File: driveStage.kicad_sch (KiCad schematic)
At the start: 45 parts

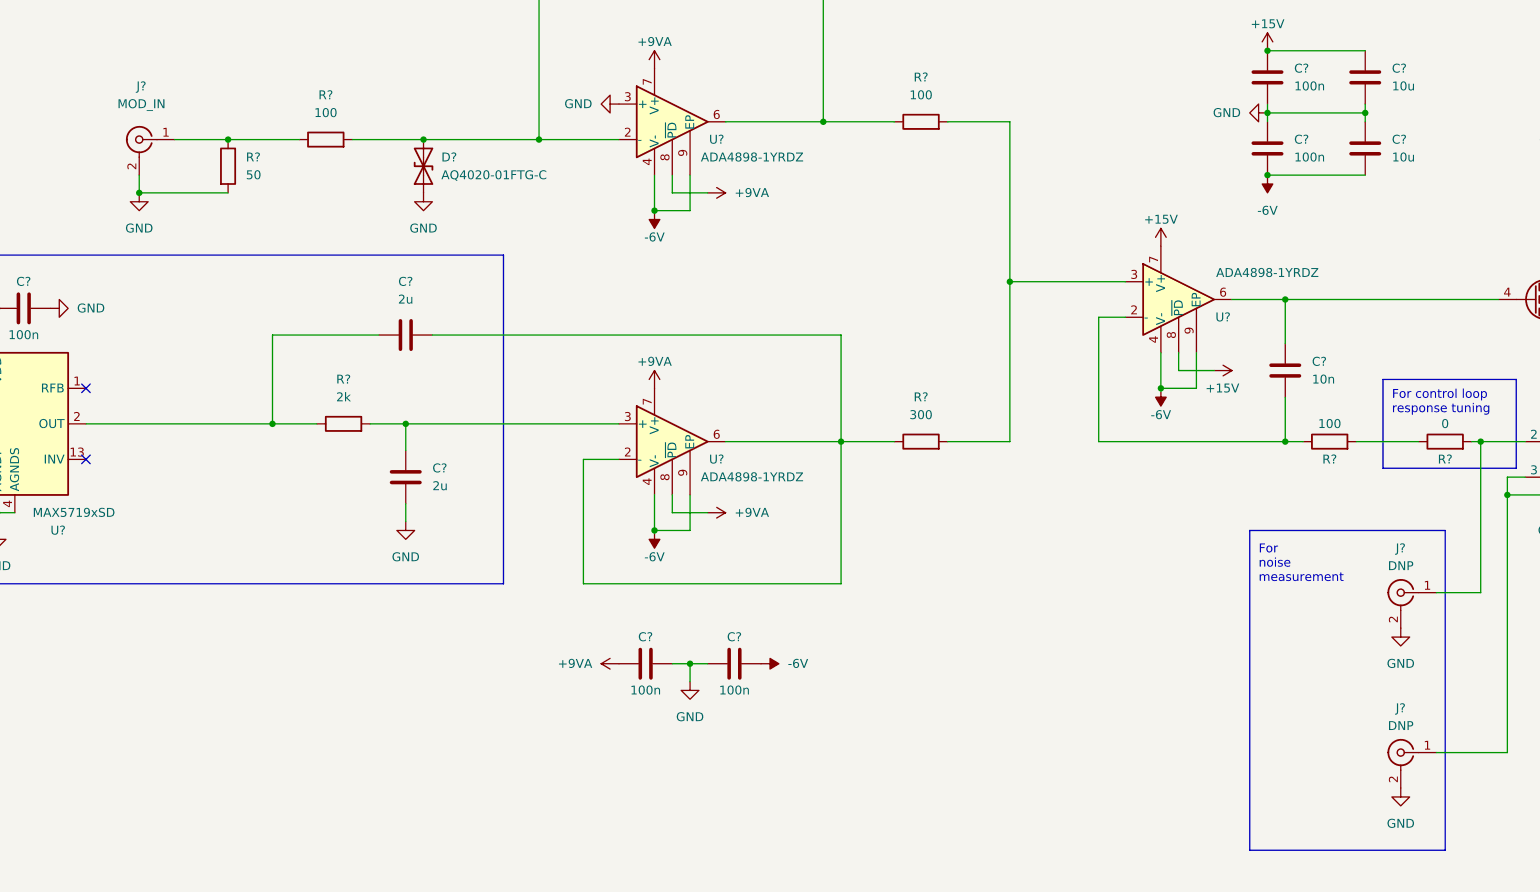
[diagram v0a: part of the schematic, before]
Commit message: add PoE
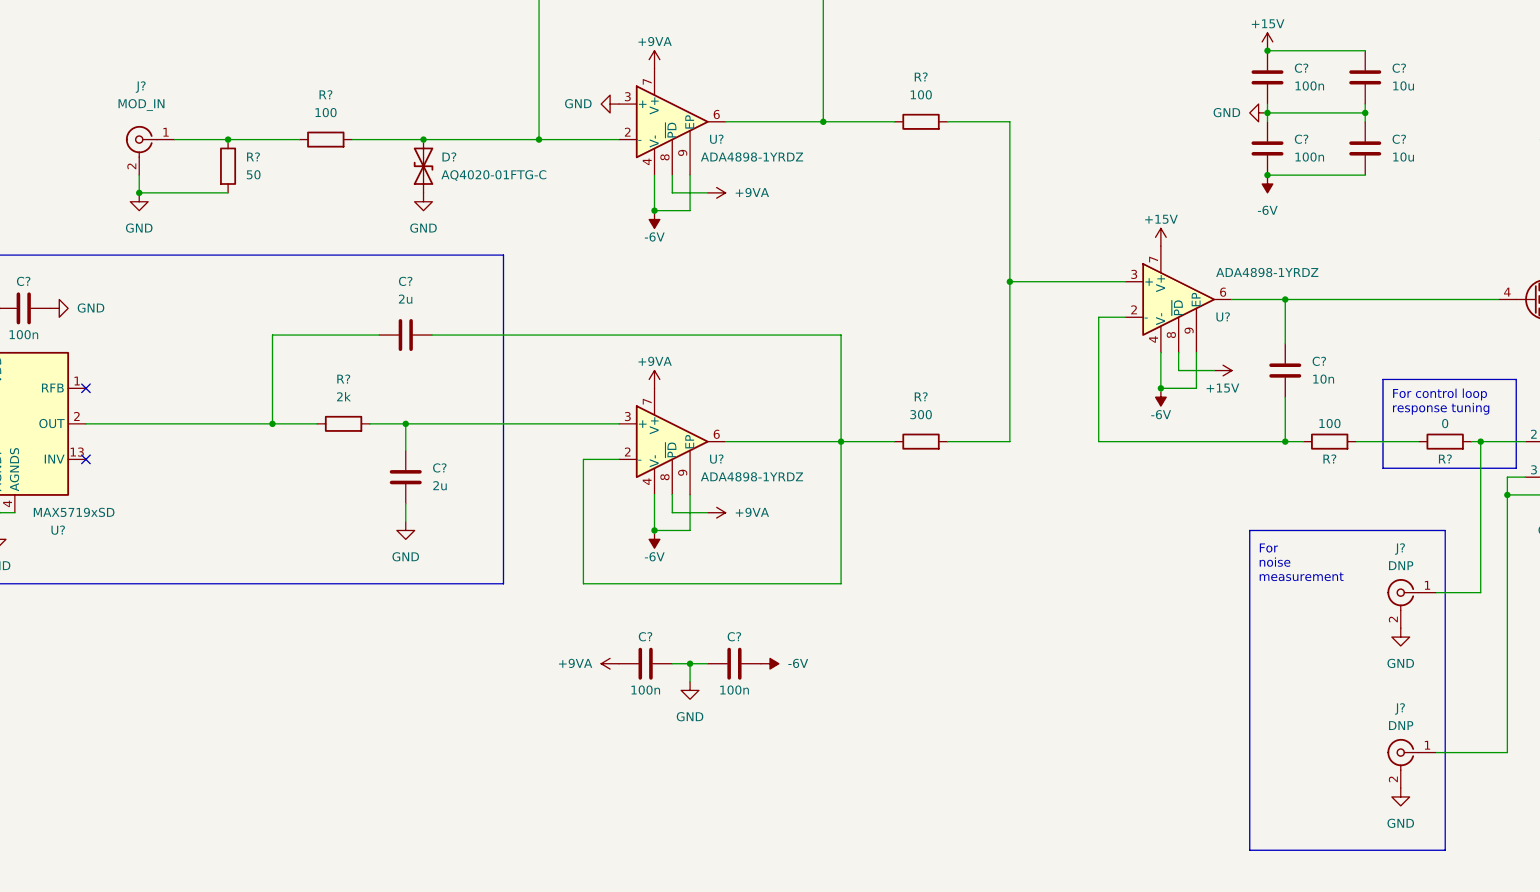
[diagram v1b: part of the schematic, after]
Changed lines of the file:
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@@
       (effects (font (size 1.27 1.27)) hide)
     )
-    (pin "1")
-    (pin "2")
-    (pin "3")
     (pin "5")
     (pin "6")
     (pin "7")
-    (pin "4")
-    (pin "8")
   )
   (symbol (lib_id "kirdy:RS8552") (at 339.09 208.28 0) (mirror y) (unit 1)
@@
     (pin "2")
     (pin "3")
-    (pin "5")
-    (pin "6")
-    (pin "7")
-    (pin "4")
-    (pin "8")
   )
   (symbol (lib_id "power:GND") (at 96.52 99.06 180) (unit 1)
@@
       (effects (font (size 1.27 1.27)) hide)
     )
-    (pin "1")
-    (pin "2")
-    (pin "3")
-    (pin "5")
-    (pin "6")
-    (pin "7")
     (pin "4")
     (pin "8")
